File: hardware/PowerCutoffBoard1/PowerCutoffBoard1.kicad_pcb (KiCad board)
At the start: 2 copper layers, 50 x 45 mm, 49 parts, among them J1 Conn_Coaxial, J2 Conn_01x03, J3 Conn_01x04, J5 Conn_01x04, J6 Conn_01x04, SW1 SW_Push, SW2 SW_Push, SW3 SW_DIP_x04, U1 STM32F303K8Tx, U2 Wio-E5, U3 3.3V, U4 MIC4427, U5 MCP2562-E-SN

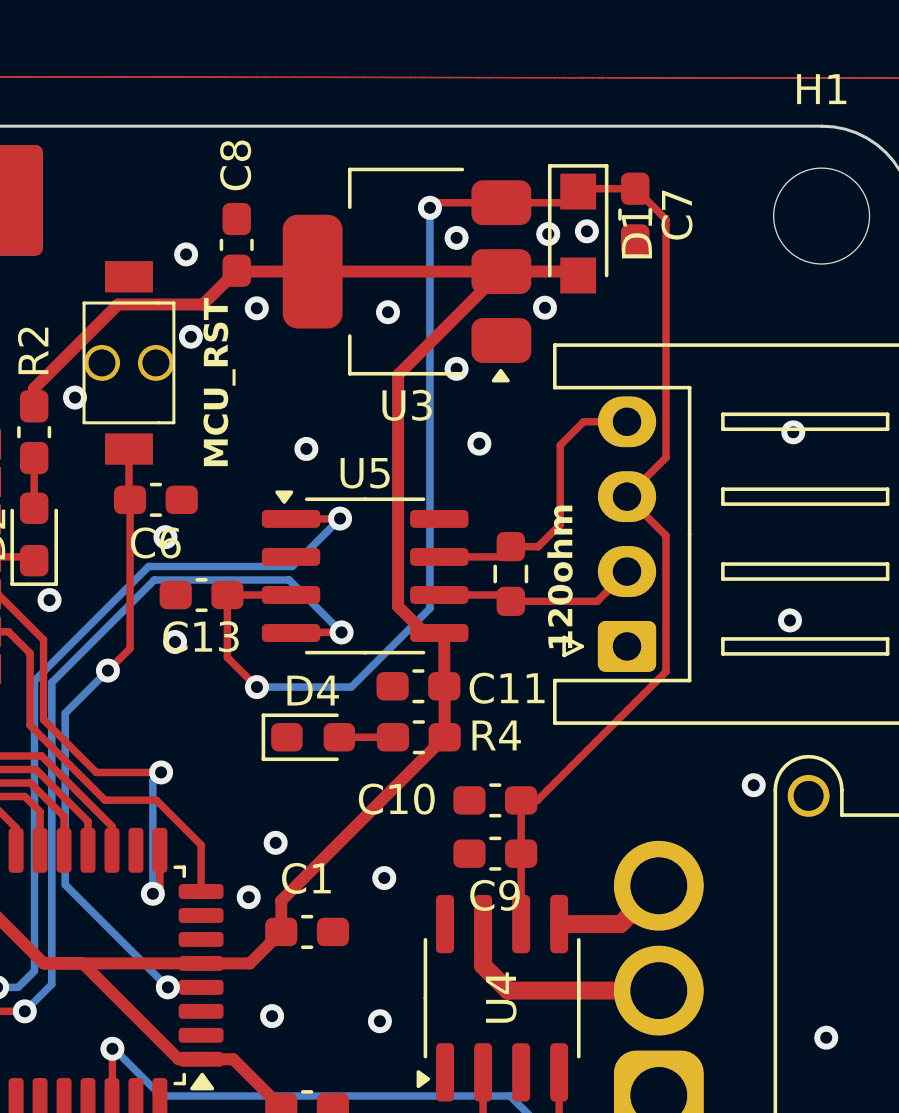
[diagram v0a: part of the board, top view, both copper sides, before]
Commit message: update
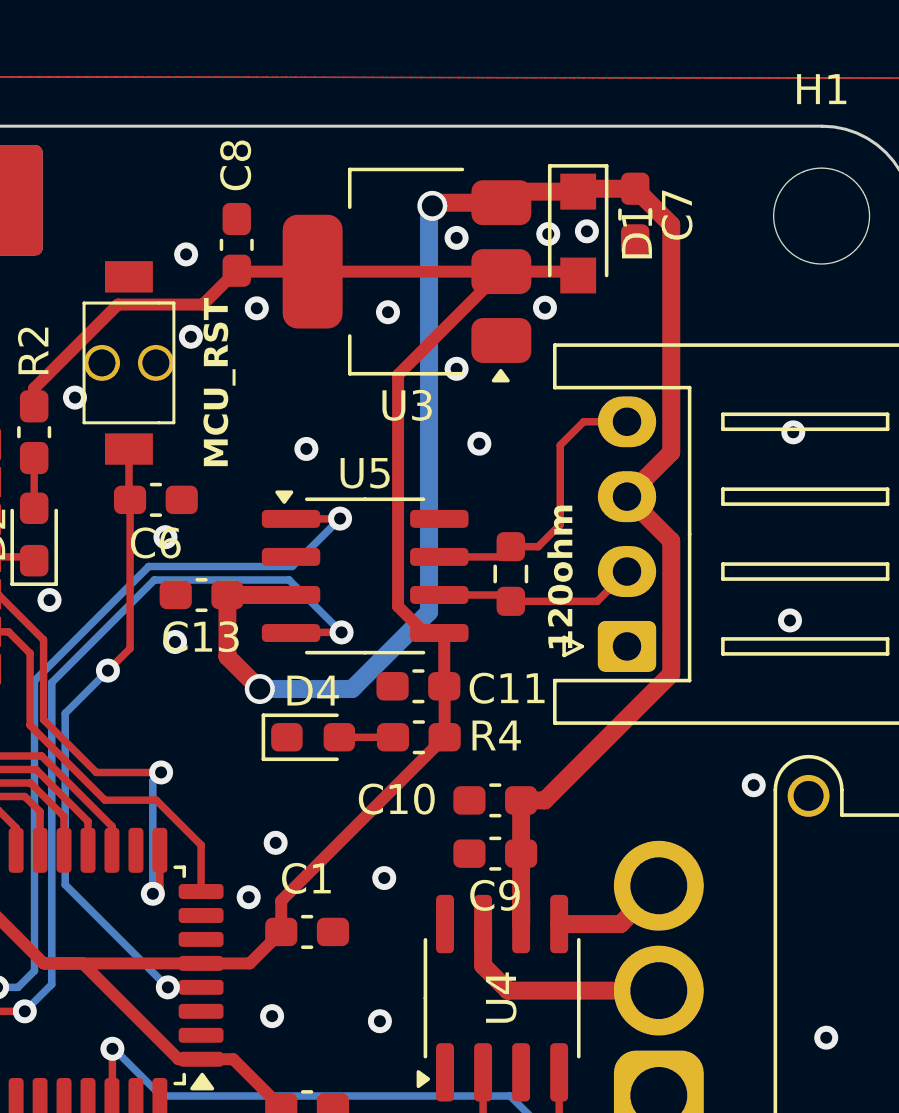
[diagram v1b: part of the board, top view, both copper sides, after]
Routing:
- net +5V: track 61.3 -> 61.9 mm
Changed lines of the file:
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@@
 	)
 	(segment
-		(start 191.78 108.1135)
-		(end 191.78 116.067)
-		(width 0.25)
+		(start 178.22 123.79)
+		(end 177.1385 122.7085)
+		(width 0.6)
 		(layer "F.Cu")
 		(net 36)
 	)
 	(segment
-		(start 184.07 107.555)
-		(end 183.9 107.725)
-		(width 0.25)
+		(start 190.754 107.0875)
+		(end 188.9465 107.0875)
+		(width 0.6)
+		(layer "F.Cu")
+		(net 36)
+	)
+	(segment
+		(start 190.754 107.0875)
+		(end 191.955 108.2885)
+		(width 0.6)
+		(layer "F.Cu")
+		(net 36)
+	)
+	(segment
+		(start 184.085 107.555)
+		(end 183.98 107.66)
+		(width 0.6)
+		(layer "F.Cu")
+		(net 36)
+	)
+	(segment
+		(start 191.955 118.844)
+		(end 191.955 123.286002)
+		(width 0.6)
+		(layer "F.Cu")
+		(net 36)
+	)
+	(segment
+		(start 186.944 127.508)
+		(end 186.944 129.286)
+		(width 0.6)
+		(layer "F.Cu")
+		(net 36)
+	)
+	(segment
+		(start 186.654 107.185)
+		(end 186.284 107.555)
+		(width 0.6)
 		(layer "F.Cu")
 		(net 36)
@@
 		(start 188.9465 107.0875)
 		(end 188.849 107.185)
-		(width 0.25)
+		(width 0.6)
 		(layer "F.Cu")
 		(net 36)
 	)
 	(segment
-		(start 186.944 127.508)
-		(end 186.944 129.286)
-		(width 0.25)
+		(start 186.944 129.286)
+		(end 186.944 131.637)
+		(width 0.6)
 		(layer "F.Cu")
 		(net 36)
 	)
 	(segment
-		(start 188.71 107.185)
-		(end 188.34 107.555)
-		(width 0.25)
+		(start 188.849 107.185)
+		(end 186.654 107.185)
+		(width 0.6)
 		(layer "F.Cu")
 		(net 36)
 	)
 	(segment
-		(start 190.754 107.0875)
-		(end 191.78 108.1135)
-		(width 0.25)
+		(start 191.955 108.2885)
+		(end 191.955 115.892)
+		(width 0.6)
 		(layer "F.Cu")
 		(net 36)
 	)
 	(segment
-		(start 190.754 107.0875)
-		(end 188.9465 107.0875)
-		(width 0.25)
-		(layer "F.Cu")
-		(net 36)
-	)
-	(segment
-		(start 188.34 107.555)
-		(end 186.284 107.555)
-		(width 0.25)
-		(layer "F.Cu")
-		(net 36)
-	)
-	(segment
-		(start 178.125 123.725)
-		(end 177.1385 122.7385)
-		(width 0.25)
-		(layer "F.Cu")
-		(net 36)
-	)
-	(segment
-		(start 187.485514 127.508)
-		(end 191.78 123.213514)
-		(width 0.25)
-		(layer "F.Cu")
-		(net 36)
-	)
-	(segment
-		(start 191.78 116.067)
+		(start 191.955 115.892)
 		(end 190.479 117.368)
-		(width 0.25)
-		(layer "F.Cu")
-		(net 36)
-	)
-	(segment
-		(start 177.1385 122.7385)
-		(end 177.1385 120.65)
-		(width 0.25)
-		(layer "F.Cu")
-		(net 36)
-	)
-	(segment
-		(start 191.78 118.669)
-		(end 190.479 117.368)
-		(width 0.25)
-		(layer "F.Cu")
-		(net 36)
-	)
-	(segment
-		(start 191.78 123.213514)
-		(end 191.78 118.669)
-		(width 0.25)
+		(width 0.6)
 		(layer "F.Cu")
 		(net 36)
@@
 	(segment
 		(start 186.284 107.555)
-		(end 184.07 107.555)
-		(width 0.25)
+		(end 184.085 107.555)
+		(width 0.6)
 		(layer "F.Cu")
 		(net 36)
 	)
 	(segment
-		(start 188.849 107.185)
-		(end 188.71 107.185)
-		(width 0.25)
+		(start 177.1385 122.7085)
+		(end 177.1385 120.65)
+		(width 0.6)
 		(layer "F.Cu")
 		(net 36)
 	)
 	(segment
-		(start 186.944 127.508)
-		(end 187.485514 127.508)
-		(width 0.25)
+		(start 190.479 117.368)
+		(end 191.955 118.844)
+		(width 0.6)
 		(layer "F.Cu")
 		(net 36)
 	)
 	(segment
-		(start 179.262 120.65)
-		(end 177.1385 120.65)
-		(width 0.25)
+		(start 191.955 123.286002)
+		(end 187.733002 127.508)
+		(width 0.6)
 		(layer "F.Cu")
 		(net 36)
 	)
 	(segment
-		(start 186.944 131.637)
-		(end 186.944 129.286)
-		(width 0.25)
+		(start 177.1385 120.65)
+		(end 179.262 120.65)
+		(width 0.6)
+		(layer "F.Cu")
+		(net 36)
+	)
+	(segment
+		(start 187.733002 127.508)
+		(end 186.944 127.508)
+		(width 0.6)
 		(layer "F.Cu")
 		(net 36)
 	)
 	(via
-		(at 183.9 107.725)
-		(size 0.8)
-		(drill 0.4)
+		(at 178.22 123.79)
+		(size 1)
+		(drill 0.7)
 		(layers "F.Cu" "B.Cu")
 		(net 36)
 	)
 	(via
-		(at 178.125 123.725)
-		(size 0.8)
-		(drill 0.4)
+		(at 183.98 107.66)
+		(size 1)
+		(drill 0.7)
 		(layers "F.Cu" "B.Cu")
 		(net 36)
 	)
 	(segment
-		(start 183.9 107.725)
-		(end 183.9 121.1)
-		(width 0.25)
+		(start 183.98 107.66)
+		(end 183.87 107.77)
+		(width 0.6)
 		(layer "B.Cu")
 		(net 36)
 	)
 	(segment
-		(start 181.275 123.725)
-		(end 178.125 123.725)
-		(width 0.25)
+		(start 183.87 121.01)
+		(end 183.87 121.22)
+		(width 0.6)
 		(layer "B.Cu")
 		(net 36)
 	)
 	(segment
-		(start 183.9 121.1)
-		(end 181.275 123.725)
-		(width 0.25)
+		(start 183.87 107.77)
+		(end 183.87 121.01)
+		(width 0.6)
 		(layer "B.Cu")
 		(net 36)
+	)
+	(segment
+		(start 183.87 121.22)
+		(end 181.38 123.71)
+		(width 0.6)
+		(layer "B.Cu")
+		(net 36)
+	)
+	(segment
+		(start 181.38 123.71)
+		(end 181.3 123.79)
+		(width 0.6)
+		(layer "B.Cu")
+		(net 36)
+	)
+	(segment
+		(start 181.3 123.79)
+		(end 178.22 123.79)
+		(width 0.6)
+		(layer "B.Cu")
+		(net 36)
